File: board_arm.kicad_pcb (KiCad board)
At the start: 2 copper layers, 314.3 x 95.2 mm, 152 parts, among them SW1 SW_SPDT, U1 STM32F072CBT6, U2 PRTR5V0U2X, U3 MCP1725-3302E_SN

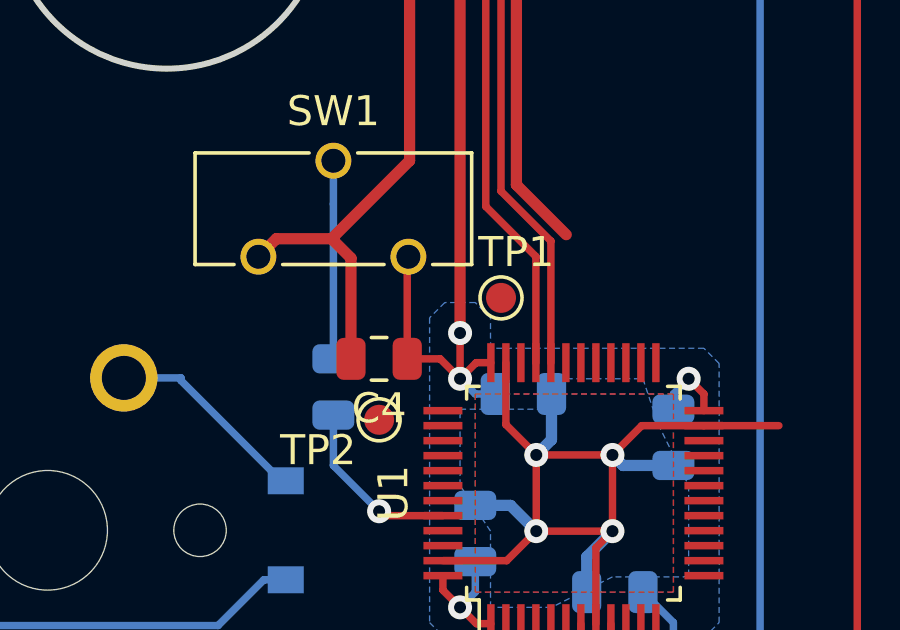
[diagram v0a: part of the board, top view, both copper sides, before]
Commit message: corrections sur les TP
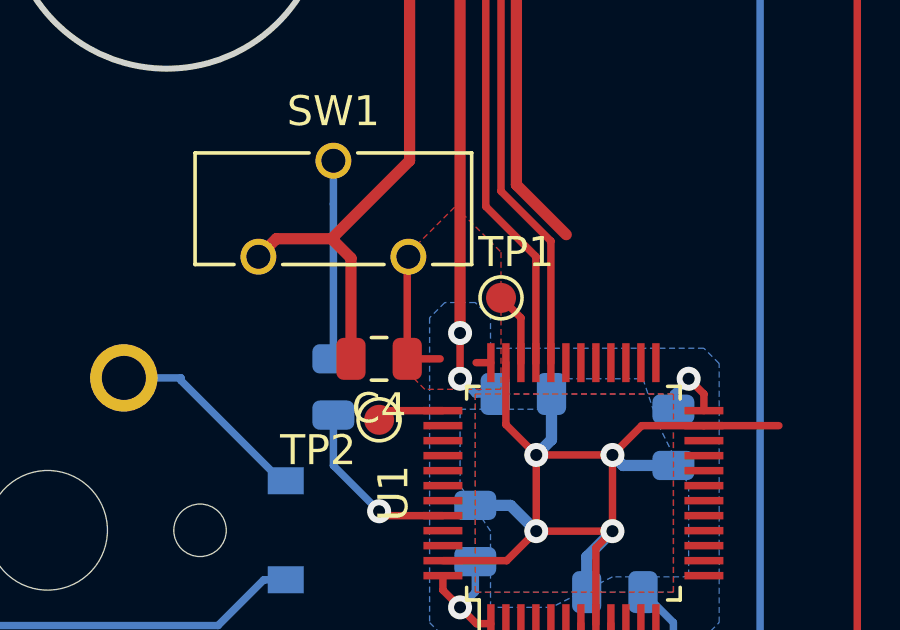
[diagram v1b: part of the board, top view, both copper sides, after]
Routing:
- net SWDIO: track 0.00 -> 2.43 mm
- net SWDCLK: track 0.00 -> 2.25 mm
- net +3V3: track 81.7 -> 80.0 mm
- added copper zone on F.Cu, net +3V3
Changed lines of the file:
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@@
     (thickness 1.6)
     (drawings 9)
-    (tracks 1056)
+    (tracks 1058)
     (zones 0)
     (modules 152)
@@
     (42 Eco1.User user hide)
     (43 Eco2.User user hide)
-    (44 Edge.Cuts user hide)
+    (44 Edge.Cuts user)
     (45 Margin user hide)
     (46 B.CrtYd user hide)
@@
   (gr_arc (start 359.56875 156.36875) (end 359.56875 158.75) (angle -90) (layer Edge.Cuts) (width 0.2))
   (gr_arc (start 359.56875 65.88125) (end 361.95 65.88125) (angle -90) (layer Edge.Cuts) (width 0.2))
-  (via (at 344.424 129.54) (size 0.8) (drill 0.4) (layers F.Cu B.Cu) (net 101))
-  (via (at 354.234482 136.299484) (size 0.8) (drill 0.4) (layers F.Cu B.Cu) (net 98))
   (via (at 352.202482 130.203484) (size 0.8) (drill 0.4) (layers F.Cu B.Cu) (net 1))
   (via (at 349.662482 127.663484) (size 0.8) (drill 0.4) (layers F.Cu B.Cu) (net 1))
   (via (at 349.662482 130.203484) (size 0.8) (drill 0.4) (layers F.Cu B.Cu) (net 1))
-  (via (at 354.742482 125.123484) (size 0.8) (drill 0.4) (layers F.Cu B.Cu) (net 98))
-  (via (at 347.122482 125.123484) (size 0.8) (drill 0.4) (layers F.Cu B.Cu) (net 98))
-  (via (at 347.122482 132.743484) (size 0.8) (drill 0.4) (layers F.Cu B.Cu) (net 98))
   (via (at 352.202482 127.663484) (size 0.8) (drill 0.4) (layers F.Cu B.Cu) (net 1))
   (segment (start 334.7432 69.6618) (end 333.8282 68.7468) (width 0.375) (layer B.Cu) (net 1))
@@
   (segment (start 337.987001 72.644) (end 337.987001 71.287001) (width 0.25) (layer B.Cu) (net 92))
   (segment (start 337.362 74.036) (end 338.002 74.676) (width 0.25) (layer B.Cu) (net 92))
+  (segment (start 338.002 74.676) (end 342.9 74.676) (width 0.25) (layer B.Cu) (net 92))
+  (segment (start 342.9 74.676) (end 343.916 74.676) (width 0.25) (layer B.Cu) (net 92))
+  (segment (start 344.37052 75.13052) (end 344.92749 75.68749) (width 0.25) (layer F.Cu) (net 92))
+  (segment (start 343.916 74.676) (end 344.37052 75.13052) (width 0.25) (layer F.Cu) (net 92))
+  (segment (start 344.92749 75.68749) (end 344.932 75.692) (width 0.25) (layer F.Cu) (net 92))
+  (segment (start 344.92749 99.05549) (end 344.92749 75.68749) (width 0.25) (layer F.Cu) (net 92))
+  (segment (start 348.488 102.616) (end 344.92749 99.05549) (width 0.25) (layer F.Cu) (net 92))
+  (segment (start 348.488 118.872) (end 348.488 102.616) (width 0.25) (layer F.Cu) (net 92))
+  (segment (start 350.150482 124.587484) (end 350.150482 120.534482) (width 0.25) (layer F.Cu) (net 92))
+  (segment (start 350.150482 120.534482) (end 348.488 118.872) (width 0.25) (layer F.Cu) (net 92))
   (segment (start 336.8982 70.6368) (end 336.804 70.731) (width 0.25) (layer B.Cu) (net 93))
   (segment (start 336.8982 69.6618) (end 336.8982 70.6368) (width 0.25) (layer B.Cu) (net 93))
@@
   (segment (start 336.804 70.731) (end 336.804 70.731) (width 0.25) (layer B.Cu) (net 93))
   (via (at 336.804 71.12) (size 0.8) (drill 0.4) (layers F.Cu B.Cu) (net 93))
+  (segment (start 337.312 70.104) (end 337.312 70.612) (width 0.25) (layer F.Cu) (net 93))
+  (segment (start 336.804 70.3604) (end 337.0604 70.104) (width 0.25) (layer F.Cu) (net 93))
+  (segment (start 336.804 71.12) (end 336.804 70.3604) (width 0.25) (layer F.Cu) (net 93))
   (via (at 341.376 73.66) (size 0.8) (drill 0.4) (layers F.Cu B.Cu) (net 94))
   (segment (start 337.8982 68.6868) (end 338.132 68.453) (width 0.25) (layer B.Cu) (net 94))
@@
   (segment (start 339.262 74.036) (end 338.636999 73.410999) (width 0.25) (layer B.Cu) (net 94))
   (segment (start 339.312 74.036) (end 339.262 74.036) (width 0.25) (layer B.Cu) (net 94))
-  (segment (start 338.002 74.676) (end 342.9 74.676) (width 0.25) (layer B.Cu) (net 92))
-  (segment (start 342.9 74.676) (end 343.916 74.676) (width 0.25) (layer B.Cu) (net 92))
-  (segment (start 344.37052 75.13052) (end 344.92749 75.68749) (width 0.25) (layer F.Cu) (net 92))
-  (segment (start 343.916 74.676) (end 344.37052 75.13052) (width 0.25) (layer F.Cu) (net 92))
-  (segment (start 344.92749 75.68749) (end 344.932 75.692) (width 0.25) (layer F.Cu) (net 92))
-  (segment (start 344.92749 99.05549) (end 344.92749 75.68749) (width 0.25) (layer F.Cu) (net 92))
-  (segment (start 348.488 102.616) (end 344.92749 99.05549) (width 0.25) (layer F.Cu) (net 92))
-  (segment (start 348.488 118.872) (end 348.488 102.616) (width 0.25) (layer F.Cu) (net 92))
-  (segment (start 350.150482 124.587484) (end 350.150482 120.534482) (width 0.25) (layer F.Cu) (net 92))
-  (segment (start 350.150482 120.534482) (end 348.488 118.872) (width 0.25) (layer F.Cu) (net 92))
-  (segment (start 337.312 70.104) (end 337.312 70.612) (width 0.25) (layer F.Cu) (net 93))
-  (segment (start 336.804 70.3604) (end 337.0604 70.104) (width 0.25) (layer F.Cu) (net 93))
-  (segment (start 336.804 71.12) (end 336.804 70.3604) (width 0.25) (layer F.Cu) (net 93))
   (segment (start 341 74.036) (end 341.376 73.66) (width 0.25) (layer B.Cu) (net 94))
   (segment (start 339.312 74.036) (end 341 74.036) (width 0.25) (layer B.Cu) (net 94))
@@
   (segment (start 339.344 70.104) (end 339.344 70.5196) (width 0.25) (layer F.Cu) (net 95))
   (segment (start 339.344 70.104) (end 339.344 71.0738) (width 0.25) (layer F.Cu) (net 95))
+  (via (at 354.234482 136.299484) (size 0.8) (drill 0.4) (layers F.Cu B.Cu) (net 98))
+  (via (at 354.742482 125.123484) (size 0.8) (drill 0.4) (layers F.Cu B.Cu) (net 98))
+  (via (at 347.122482 125.123484) (size 0.8) (drill 0.4) (layers F.Cu B.Cu) (net 98))
+  (via (at 347.122482 132.743484) (size 0.8) (drill 0.4) (layers F.Cu B.Cu) (net 98))
   (segment (start 341.5284 77.089) (end 341.5284 75.819) (width 0.508) (layer F.Cu) (net 98))
   (segment (start 340.8172 77.089) (end 341.5284 77.089) (width 0.25) (layer F.Cu) (net 98))
@@
   (segment (start 342.2396 77.089) (end 341.5284 77.089) (width 0.375) (layer F.Cu) (net 98))
   (segment (start 343.8906 78.74) (end 342.2396 77.089) (width 0.375) (layer F.Cu) (net 98))
-  (segment (start 346.458998 124.46) (end 347.122482 125.123484) (width 0.25) (layer F.Cu) (net 98))
   (segment (start 345.3615 124.46) (end 346.458998 124.46) (width 0.25) (layer F.Cu) (net 98))
   (segment (start 347.122482 125.123484) (end 347.122482 123.599484) (width 0.25) (layer F.Cu) (net 98))
-  (segment (start 347.658482 124.587484) (end 347.122482 125.123484) (width 0.25) (layer F.Cu) (net 98))
   (segment (start 348.150482 124.587484) (end 347.658482 124.587484) (width 0.25) (layer F.Cu) (net 98))
   (segment (start 343.8906 78.74) (end 343.8906 99.5426) (width 0.375) (layer F.Cu) (net 98))
@@
   (segment (start 339.852 79.3242) (end 340.8172 78.359) (width 0.25) (layer F.Cu) (net 100))
   (segment (start 339.852 82.139) (end 339.852 79.3242) (width 0.25) (layer F.Cu) (net 100))
+  (via (at 344.424 129.54) (size 0.8) (drill 0.4) (layers F.Cu B.Cu) (net 101))
   (segment (start 344.571484 129.687484) (end 344.424 129.54) (width 0.25) (layer F.Cu) (net 101))
   (segment (start 346.550482 129.687484) (end 344.571484 129.687484) (width 0.25) (layer F.Cu) (net 101))
   (segment (start 342.9 128.016) (end 344.424 129.54) (width 0.25) (layer B.Cu) (net 101))
   (segment (start 342.9 126.335) (end 342.9 128.016) (width 0.25) (layer B.Cu) (net 101))
+  (segment (start 349.150482 123.090482) (end 348.488 122.428) (width 0.25) (layer F.Cu) (net 127))
+  (segment (start 349.150482 124.587484) (end 349.150482 123.090482) (width 0.25) (layer F.Cu) (net 127))
+  (segment (start 344.728516 126.187484) (end 344.424 126.492) (width 0.25) (layer F.Cu) (net 128))
+  (segment (start 346.550482 126.187484) (end 344.728516 126.187484) (width 0.25) (layer F.Cu) (net 128))
   (zone (net 1) (net_name GND) (layer B.Cu) (hatch edge 0.508)
     (connect_pads (clearance 0.381))
@@
       )
     )
+  )
+  (zone (net 98) (net_name +3V3) (layer F.Cu) (hatch edge 0.508)
+    (connect_pads (clearance 0.381))
+    (min_thickness 0.254)
+    (fill yes (arc_segments 16) (thermal_gap 0.508) (thermal_bridge_width 0.508))
+    (polygon
+      (pts
+        (xy 345.44 120.904) (xy 346.964 119.38) (xy 348.488 120.904) (xy 348.488 125.476) (xy 345.948 125.476)
+        (xy 345.44 124.968)
+      )
+    )
